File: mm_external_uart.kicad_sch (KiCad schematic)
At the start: 0 parts

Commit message: fin tp2
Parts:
- added J6: Conn_01x04, Connector_PinHeader_2.54mm:PinHeader_1x04_P2.54mm_Vertical, symbol Connector_Generic:Conn_01x04
- added R9: 100 Ohms, symbol Device:R
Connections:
- new net: J6.4 (Pin_4), R9.2
- new net GND: J6.2 (Pin_2)
- new net RX: R9.1
- new net TX: J6.3 (Pin_3)
- new net VBATT: J6.1 (Pin_1)
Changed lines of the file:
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@@
 (kicad_sch (version 20230121) (generator eeschema)
   (paper "A4")
+  (wire (pts (xy 146.05 85.09) (xy 161.29 85.09))
+    (stroke (width 0) (type default))
+  )
+  (wire (pts (xy 142.24 92.71) (xy 153.67 92.71))
+    (stroke (width 0) (type default))
+  )
+  (wire (pts (xy 146.05 90.17) (xy 161.29 90.17))
+    (stroke (width 0) (type default))
+  )
+  (wire (pts (xy 146.05 87.63) (xy 161.29 87.63))
+    (stroke (width 0) (type default))
+  )
+  (hierarchical_label "VBATT" (shape input) (at 146.05 85.09 180) (fields_autoplaced)
+    (effects (font (size 1.27 1.27)) (justify right))
+  )
+  (hierarchical_label "TX" (shape input) (at 146.05 90.17 0) (fields_autoplaced)
+    (effects (font (size 1.27 1.27)) (justify left))
+  )
+  (hierarchical_label "GND" (shape output) (at 146.05 87.63 180) (fields_autoplaced)
+    (effects (font (size 1.27 1.27)) (justify right))
+  )
+  (hierarchical_label "RX" (shape output) (at 142.24 92.71 0) (fields_autoplaced)
+    (effects (font (size 1.27 1.27)) (justify left))
+  )
+  (symbol (lib_id "Device:R") (at 157.48 92.71 90) (mirror x) (unit 1)
+    (in_bom yes) (on_board yes) (dnp no)
+    (property "Reference" "R9" (at 157.48 96.52 90)
+      (effects (font (size 1.27 1.27)))
+    )
+    (property "Value" "100 Ohms" (at 160.02 99.06 90)
+      (effects (font (size 1.27 1.27)) (justify left))
+    )
+    (property "Footprint" "" (at 157.48 90.932 90)
+      (effects (font (size 1.27 1.27)) hide)
+    )
+    (property "Datasheet" "~" (at 157.48 92.71 0)
+      (effects (font (size 1.27 1.27)) hide)
+    )
+    (pin "2")
+    (pin "1")
+    (instances
+      (project "minimouse"
+        (path "/d8fa4cba-2469-4231-847f-065b6b829f44/d17bb1c7-f68a-465e-9a17-5858ef86fc30"
+          (reference "R9") (unit 1)
+        )
+      )
+    )
+  )
+  (symbol (lib_id "Connector_Generic:Conn_01x04") (at 166.37 87.63 0) (unit 1)
+    (in_bom yes) (on_board yes) (dnp no) (fields_autoplaced)
+    (property "Reference" "J6" (at 168.91 87.63 0)
+      (effects (font (size 1.27 1.27)) (justify left))
+    )
+    (property "Value" "Conn_01x04" (at 168.91 90.17 0)
+      (effects (font (size 1.27 1.27)) (justify left))
+    )
+    (property "Footprint" "Connector_PinHeader_2.54mm:PinHeader_1x04_P2.54mm_Vertical" (at 166.37 87.63 0)
+      (effects (font (size 1.27 1.27)) hide)
+    )
+    (property "Datasheet" "~" (at 166.37 87.63 0)
+      (effects (font (size 1.27 1.27)) hide)
+    )
+    (pin "4")
+    (pin "3")
+    (pin "2")
+    (pin "1")
+    (instances
+      (project "minimouse"
+        (path "/d8fa4cba-2469-4231-847f-065b6b829f44/d17bb1c7-f68a-465e-9a17-5858ef86fc30"
+          (reference "J6") (unit 1)
+        )
+      )
+    )
+  )
 )

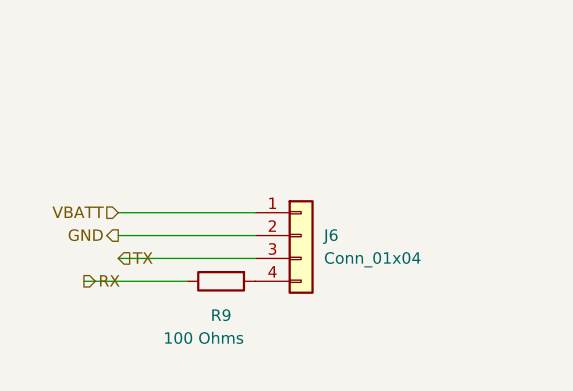
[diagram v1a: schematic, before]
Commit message: TP
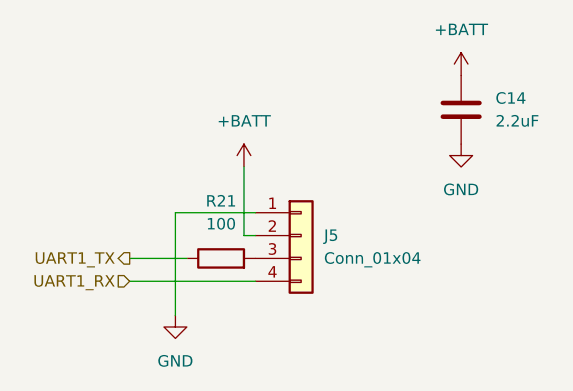
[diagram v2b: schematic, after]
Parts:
- removed R9: 100 Ohms, symbol Device:R
- added C14: 2.2uF, Capacitor_SMD:C_0603_1608Metric, symbol Device:C
- added R21: 100, Resistor_SMD:R_0603_1608Metric, symbol Device:R
- renumbered J6 to J5
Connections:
- net VBATT is gone; now on net GND: J5.1 (Pin_1)
- net GND: now also C14.2; no longer J5.2 (Pin_2)
- net UART1_RX: now reaches J5.4 (Pin_4)
- net TX: no longer names the net of J5.3 (Pin_3)
- net TX: now also R21.2
- new net +BATT: C14.1, J5.2 (Pin_2)
- new net UART1_TX: R21.1
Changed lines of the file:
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@@
 (kicad_sch (version 20230121) (generator eeschema)
   (paper "A4")
-  (wire (pts (xy 146.05 85.09) (xy 161.29 85.09))
+  (wire (pts (xy 160.02 87.63) (xy 160.02 80.01))
     (stroke (width 0) (type default))
   )
-  (wire (pts (xy 142.24 92.71) (xy 153.67 92.71))
+  (wire (pts (xy 147.32 90.17) (xy 153.67 90.17))
     (stroke (width 0) (type default))
   )
-  (wire (pts (xy 146.05 90.17) (xy 161.29 90.17))
+  (wire (pts (xy 152.4 85.09) (xy 152.4 96.52))
     (stroke (width 0) (type default))
   )
-  (wire (pts (xy 146.05 87.63) (xy 161.29 87.63))
+  (wire (pts (xy 161.29 85.09) (xy 152.4 85.09))
     (stroke (width 0) (type default))
   )
-  (hierarchical_label "VBATT" (shape input) (at 146.05 85.09 180) (fields_autoplaced)
+  (wire (pts (xy 161.29 87.63) (xy 160.02 87.63))
+    (stroke (width 0) (type default))
+  )
+  (wire (pts (xy 147.32 92.71) (xy 161.29 92.71))
+    (stroke (width 0) (type default))
+  )
+  (hierarchical_label "UART1_TX" (shape output) (at 147.32 90.17 180) (fields_autoplaced)
     (effects (font (size 1.27 1.27)) (justify right))
   )
-  (hierarchical_label "TX" (shape input) (at 146.05 90.17 0) (fields_autoplaced)
-    (effects (font (size 1.27 1.27)) (justify left))
-  )
-  (hierarchical_label "GND" (shape output) (at 146.05 87.63 180) (fields_autoplaced)
+  (hierarchical_label "UART1_RX" (shape input) (at 147.32 92.71 180) (fields_autoplaced)
     (effects (font (size 1.27 1.27)) (justify right))
   )
-  (hierarchical_label "RX" (shape output) (at 142.24 92.71 0) (fields_autoplaced)
-    (effects (font (size 1.27 1.27)) (justify left))
-  )
-  (symbol (lib_id "Device:R") (at 157.48 92.71 90) (mirror x) (unit 1)
-    (in_bom yes) (on_board yes) (dnp no)
-    (property "Reference" "R9" (at 157.48 96.52 90)
+  (symbol (lib_id "power:+BATT") (at 184.15 69.85 0) (unit 1)
+    (in_bom yes) (on_board yes) (dnp no) (fields_autoplaced)
+    (property "Reference" "#PWR032" (at 184.15 73.66 0)
+      (effects (font (size 1.27 1.27)) hide)
+    )
+    (property "Value" "+BATT" (at 184.15 64.77 0)
       (effects (font (size 1.27 1.27)))
     )
-    (property "Value" "100 Ohms" (at 160.02 99.06 90)
+    (property "Footprint" "" (at 184.15 69.85 0)
+      (effects (font (size 1.27 1.27)) hide)
+    )
+    (property "Datasheet" "" (at 184.15 69.85 0)
+      (effects (font (size 1.27 1.27)) hide)
+    )
+    (pin "1")
+    (instances
+      (project "tp2"
+        (path "/d8fa4cba-2469-4231-847f-065b6b829f44/d17bb1c7-f68a-465e-9a17-5858ef86fc30"
+          (reference "#PWR032") (unit 1)
+        )
+      )
+    )
+  )
+  (symbol (lib_id "power:GND") (at 184.15 77.47 0) (unit 1)
+    (in_bom yes) (on_board yes) (dnp no) (fields_autoplaced)
+    (property "Reference" "#PWR033" (at 184.15 83.82 0)
+      (effects (font (size 1.27 1.27)) hide)
+    )
+    (property "Value" "GND" (at 184.15 82.55 0)
+      (effects (font (size 1.27 1.27)))
+    )
+    (property "Footprint" "" (at 184.15 77.47 0)
+      (effects (font (size 1.27 1.27)) hide)
+    )
+    (property "Datasheet" "" (at 184.15 77.47 0)
+      (effects (font (size 1.27 1.27)) hide)
+    )
+    (pin "1")
+    (instances
+      (project "tp2"
+        (path "/d8fa4cba-2469-4231-847f-065b6b829f44/d17bb1c7-f68a-465e-9a17-5858ef86fc30"
+          (reference "#PWR033") (unit 1)
+        )
+      )
+    )
+  )
+  (symbol (lib_id "power:+BATT") (at 160.02 80.01 0) (unit 1)
+    (in_bom yes) (on_board yes) (dnp no) (fields_autoplaced)
+    (property "Reference" "#PWR031" (at 160.02 83.82 0)
+      (effects (font (size 1.27 1.27)) hide)
+    )
+    (property "Value" "+BATT" (at 160.02 74.93 0)
+      (effects (font (size 1.27 1.27)))
+    )
+    (property "Footprint" "" (at 160.02 80.01 0)
+      (effects (font (size 1.27 1.27)) hide)
+    )
+    (property "Datasheet" "" (at 160.02 80.01 0)
+      (effects (font (size 1.27 1.27)) hide)
+    )
+    (pin "1")
+    (instances
+      (project "tp2"
+        (path "/d8fa4cba-2469-4231-847f-065b6b829f44/d17bb1c7-f68a-465e-9a17-5858ef86fc30"
+          (reference "#PWR031") (unit 1)
+        )
+      )
+    )
+  )
+  (symbol (lib_id "power:GND") (at 152.4 96.52 0) (unit 1)
+    (in_bom yes) (on_board yes) (dnp no) (fields_autoplaced)
+    (property "Reference" "#PWR030" (at 152.4 102.87 0)
+      (effects (font (size 1.27 1.27)) hide)
+    )
+    (property "Value" "GND" (at 152.4 101.6 0)
+      (effects (font (size 1.27 1.27)))
+    )
+    (property "Footprint" "" (at 152.4 96.52 0)
+      (effects (font (size 1.27 1.27)) hide)
+    )
+    (property "Datasheet" "" (at 152.4 96.52 0)
+      (effects (font (size 1.27 1.27)) hide)
+    )
+    (pin "1")
+    (instances
+      (project "tp2"
+        (path "/d8fa4cba-2469-4231-847f-065b6b829f44/d17bb1c7-f68a-465e-9a17-5858ef86fc30"
+          (reference "#PWR030") (unit 1)
+        )
+      )
+    )
+  )
+  (symbol (lib_id "Device:C") (at 184.15 73.66 0) (unit 1)
+    (in_bom yes) (on_board yes) (dnp no) (fields_autoplaced)
+    (property "Reference" "C14" (at 187.96 72.39 0)
       (effects (font (size 1.27 1.27)) (justify left))
     )
-    (property "Footprint" "" (at 157.48 90.932 90)
+    (property "Value" "2.2uF" (at 187.96 74.93 0)
+      (effects (font (size 1.27 1.27)) (justify left))
+    )
+    (property "Footprint" "Capacitor_SMD:C_0603_1608Metric" (at 185.1152 77.47 0)
       (effects (font (size 1.27 1.27)) hide)
     )
-    (property "Datasheet" "~" (at 157.48 92.71 0)
+    (property "Datasheet" "~" (at 184.15 73.66 0)
       (effects (font (size 1.27 1.27)) hide)
     )
+    (pin "1")
     (pin "2")
-    (pin "1")
     (instances
-      (project "minimouse"
+      (project "tp2"
         (path "/d8fa4cba-2469-4231-847f-065b6b829f44/d17bb1c7-f68a-465e-9a17-5858ef86fc30"
-          (reference "R9") (unit 1)
+          (reference "C14") (unit 1)
         )
       )
@@
   (symbol (lib_id "Connector_Generic:Conn_01x04") (at 166.37 87.63 0) (unit 1)
     (in_bom yes) (on_board yes) (dnp no) (fields_autoplaced)
-    (property "Reference" "J6" (at 168.91 87.63 0)
+    (property "Reference" "J5" (at 168.91 87.63 0)
       (effects (font (size 1.27 1.27)) (justify left))
     )
@@
     (pin "1")
     (instances
-      (project "minimouse"
+      (project "tp2"
         (path "/d8fa4cba-2469-4231-847f-065b6b829f44/d17bb1c7-f68a-465e-9a17-5858ef86fc30"
-          (reference "J6") (unit 1)
+          (reference "J5") (unit 1)
         )
       )
+    )
+  )
+  (symbol (lib_id "Device:R") (at 157.48 90.17 90) (unit 1)
+    (in_bom yes) (on_board yes) (dnp no) (fields_autoplaced)
+    (property "Reference" "R21" (at 157.48 83.82 90)
+      (effects (font (size 1.27 1.27)))
+    )
+    (property "Value" "100" (at 157.48 86.36 90)
+      (effects (font (size 1.27 1.27)))
+    )
+    (property "Footprint" "Resistor_SMD:R_0603_1608Metric" (at 157.48 91.948 90)
+      (effects (font (size 1.27 1.27)) hide)
+    )
+    (property "Datasheet" "~" (at 157.48 90.17 0)
+      (effects (font (size 1.27 1.27)) hide)
+    )
+    (pin "1")
+    (pin "2")
+    (instances
+      (project "tp2"
+        (path "/d8fa4cba-2469-4231-847f-065b6b829f44/d17bb1c7-f68a-465e-9a17-5858ef86fc30"
+          (reference "R21") (unit 1)
+        )
+      )
